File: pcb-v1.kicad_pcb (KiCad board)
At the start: 2 copper layers, 11 parts, among them J1 Conn_01x03_Socket, J10 Screw_Terminal_01x02, J2 Conn_01x03_Socket, J3 Conn_01x03_Socket, J4 Conn_01x03_Socket, J5 Conn_01x03_Socket, J6 Conn_01x03_Socket, J7 Conn_01x08_Socket, J8 Conn_01x04_Socket, J9 Screw_Terminal_01x06

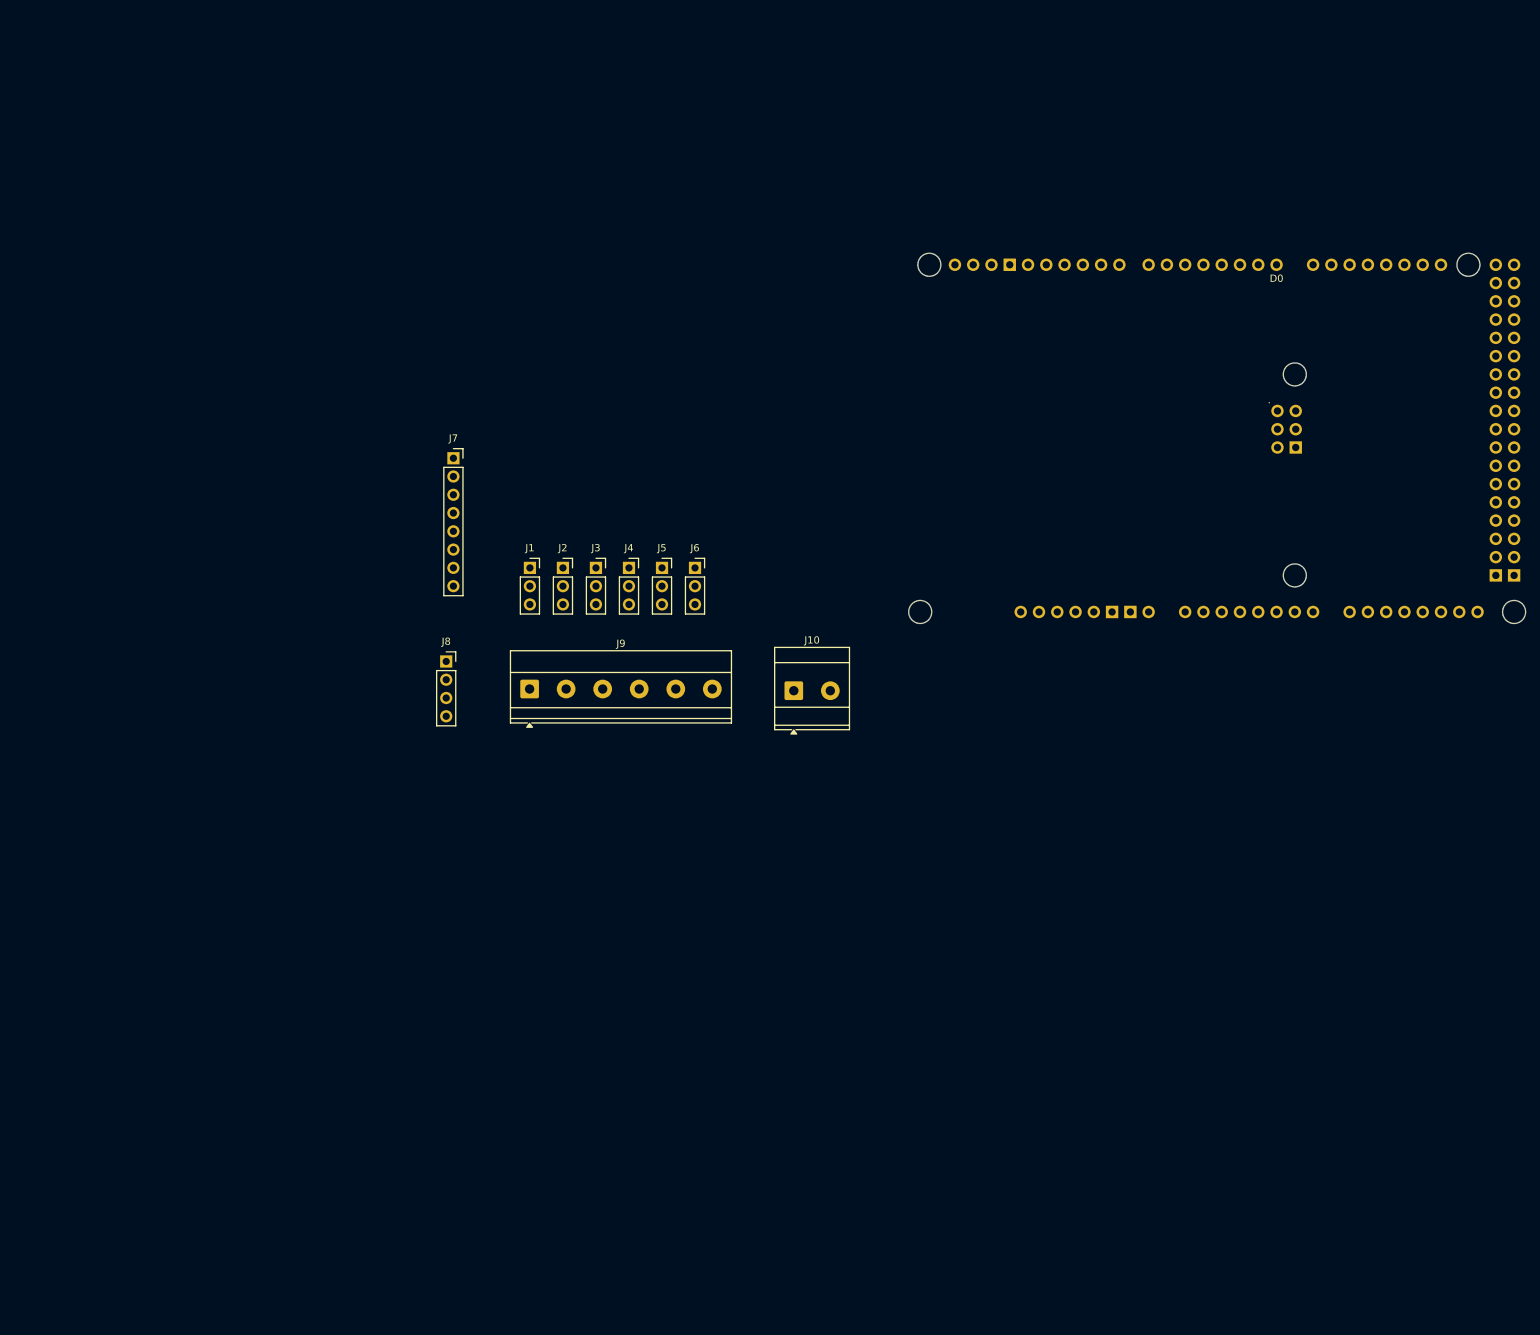
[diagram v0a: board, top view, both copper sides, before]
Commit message: before routing
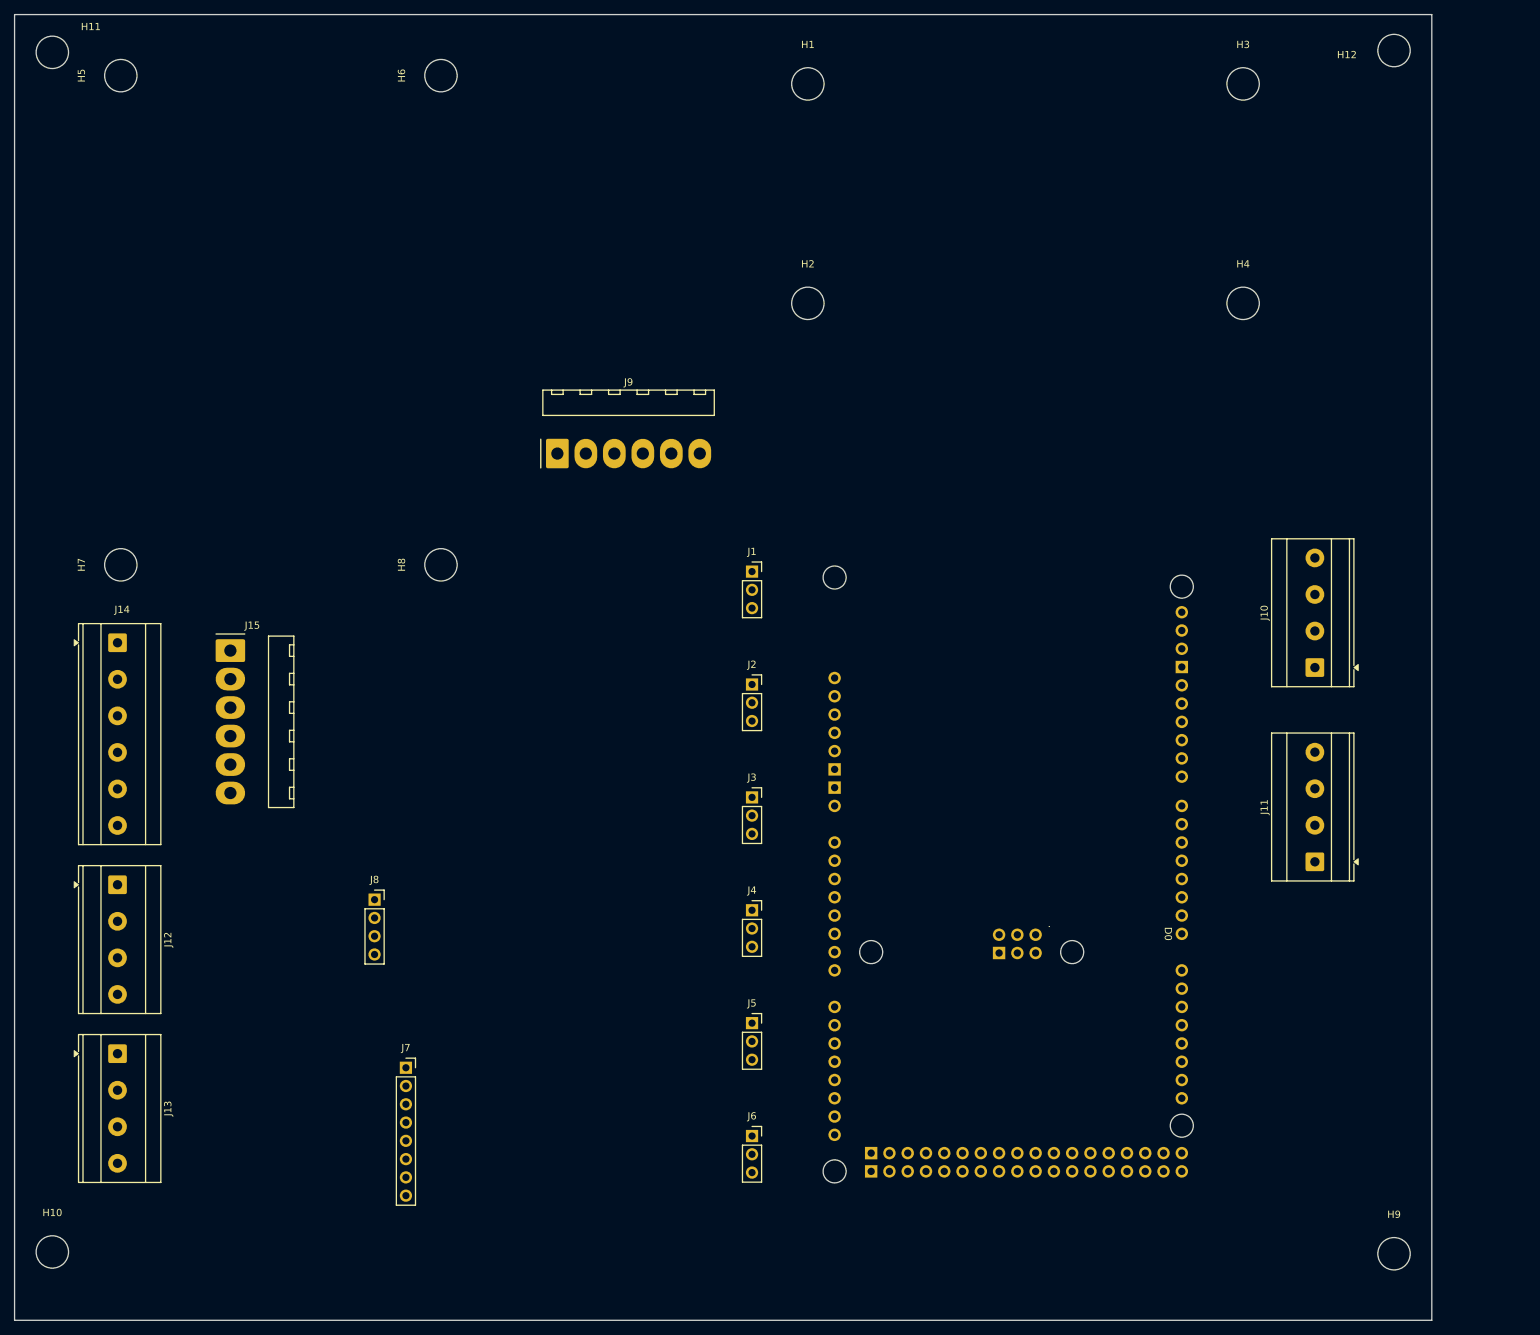
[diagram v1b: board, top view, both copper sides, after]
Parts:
- added H1: MountingHole, MountingHole:MountingHole_4.5mm, F.Cu at (165.3, 21.6)
- added H10: MountingHole, MountingHole:MountingHole_4.5mm, F.Cu at (60.2, 184.0)
- added H11: MountingHole, MountingHole:MountingHole_4.5mm, F.Cu at (60.2, 17.2)
- added H12: MountingHole, MountingHole:MountingHole_4.5mm, F.Cu at (246.8, 17.0)
- added H2: MountingHole, MountingHole:MountingHole_4.5mm, F.Cu at (165.3, 52.1)
- added H3: MountingHole, MountingHole:MountingHole_4.5mm, F.Cu at (225.8, 21.6)
- added H4: MountingHole, MountingHole:MountingHole_4.5mm, F.Cu at (225.8, 52.1)
- added H5: MountingHole, MountingHole:MountingHole_4.5mm, F.Cu at (69.8, 20.5)
- added H6: MountingHole, MountingHole:MountingHole_4.5mm, F.Cu at (114.3, 20.5)
- added H7: MountingHole, MountingHole:MountingHole_4.5mm, F.Cu at (69.8, 88.5)
- added H8: MountingHole, MountingHole:MountingHole_4.5mm, F.Cu at (114.3, 88.5)
- added H9: MountingHole, MountingHole:MountingHole_4.5mm, F.Cu at (246.8, 184.2)
- added J11: Screw_Terminal_01x04, TerminalBlock_Phoenix:TerminalBlock_Phoenix_MKDS-3-4-5.08_1x04_P5.08mm_Horizontal, F.Cu at (235.8, 129.8)
- added J12: Screw_Terminal_01x04, TerminalBlock_Phoenix:TerminalBlock_Phoenix_MKDS-3-4-5.08_1x04_P5.08mm_Horizontal, F.Cu at (69.3, 133.0)
- added J13: Screw_Terminal_01x04, TerminalBlock_Phoenix:TerminalBlock_Phoenix_MKDS-3-4-5.08_1x04_P5.08mm_Horizontal, F.Cu at (69.3, 156.4)
- added J14: Screw_Terminal_01x06, TerminalBlock_Phoenix:TerminalBlock_Phoenix_MKDS-3-6-5.08_1x06_P5.08mm_Horizontal, F.Cu at (69.3, 99.3)
- added J15: Conn_01x06_Pin, Connector_Molex:Molex_KK-396_A-41792-0006_1x06_P3.96mm_Horizontal, F.Cu at (85.0, 100.4)
- J10: value Screw_Terminal_01x02 -> Screw_Terminal_01x04; footprint TerminalBlock_Phoenix:TerminalBlock_Phoenix_MKDS-3-2-5.08_1x02_P5.08mm_Horizontal -> TerminalBlock_Phoenix:TerminalBlock_Phoenix_MKDS-3-4-5.08_1x04_P5.08mm_Horizontal
- J9: value Screw_Terminal_01x06 -> Conn_01x06_Pin; footprint TerminalBlock_Phoenix:TerminalBlock_Phoenix_MKDS-1,5-6-5.08_1x06_P5.08mm_Horizontal -> Connector_Molex:Molex_KK-396_A-41792-0006_1x06_P3.96mm_Horizontal
- moved J7 85.0 mm to (109.4, 158.4)
- moved J6 79.4 mm to (157.5, 167.9)
- moved J10 72.5 mm to (235.8, 102.8), turned to 90 degrees
- moved J5 64.5 mm to (157.5, 152.2)
- moved J4 50.6 mm to (157.5, 136.5)
- moved J3 38.6 mm to (157.5, 120.8)
- moved J8 34.6 mm to (105.0, 135.0)
- moved J9 33.0 mm to (130.4, 73.0)
- moved J1 30.9 mm to (157.5, 89.4)
- moved J2 30.9 mm to (157.5, 105.1)
- moved A1 21.3 mm to (166.4, 76.3), turned to -90 degrees
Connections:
- A1 pad D10: unconnected-(A1-PadD10) -> Net-(J9-Pin_6)
- A1 pad D7: Net-(J9-Pin_1) -> Net-(J9-Pin_3)
- A1 pad D8: Net-(J9-Pin_2) -> Net-(J9-Pin_4)
- A1 pad D9: unconnected-(A1-PadD9) -> Net-(J9-Pin_5)
- J10 pad 2: GND -> /VIN
- J9 pad 1: Net-(J9-Pin_1) -> /5VDC
- J9 pad 2: Net-(J9-Pin_2) -> GND
- J9 pad 3: unconnected-(J9-Pin_3-Pad3) -> Net-(J9-Pin_3)
- J9 pad 4: GND -> Net-(J9-Pin_4)
- J9 pad 5: /5VDC -> Net-(J9-Pin_5)
- J9 pad 6: GND -> Net-(J9-Pin_6)
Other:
- board outline added: 197 x 181.5 mm
- board text added: "Accerelator"
- board text added: "GPS Module"
- board text added: "Relay Module"
- board text added: "Step Down Module"
- board text added: "voltage sensor"
